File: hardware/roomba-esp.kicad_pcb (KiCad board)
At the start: 2 copper layers, 45 x 32.5 mm, 7 parts, among them P1 CONN_01X07, P2 CONN_02X10, U1 ESP-12E, U2 LM2596_module

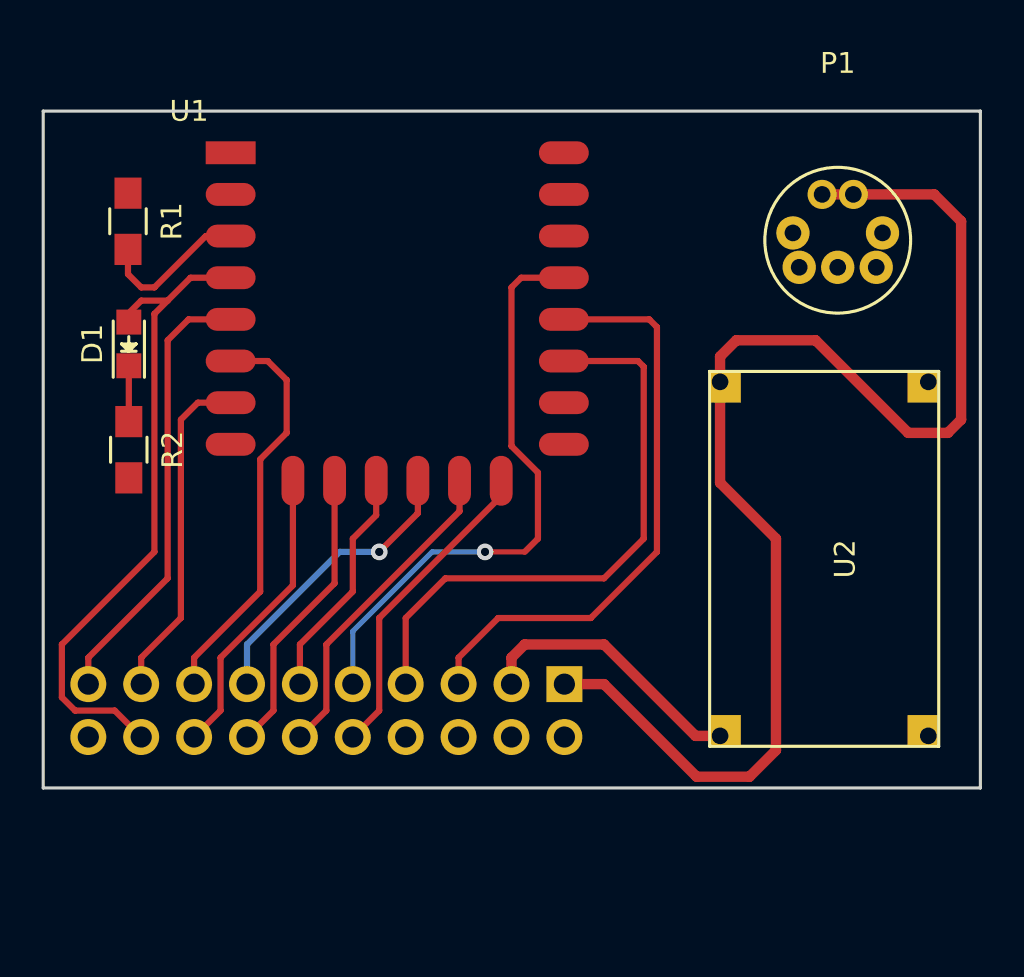
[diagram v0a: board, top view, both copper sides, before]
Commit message: finalised rev0 pcb
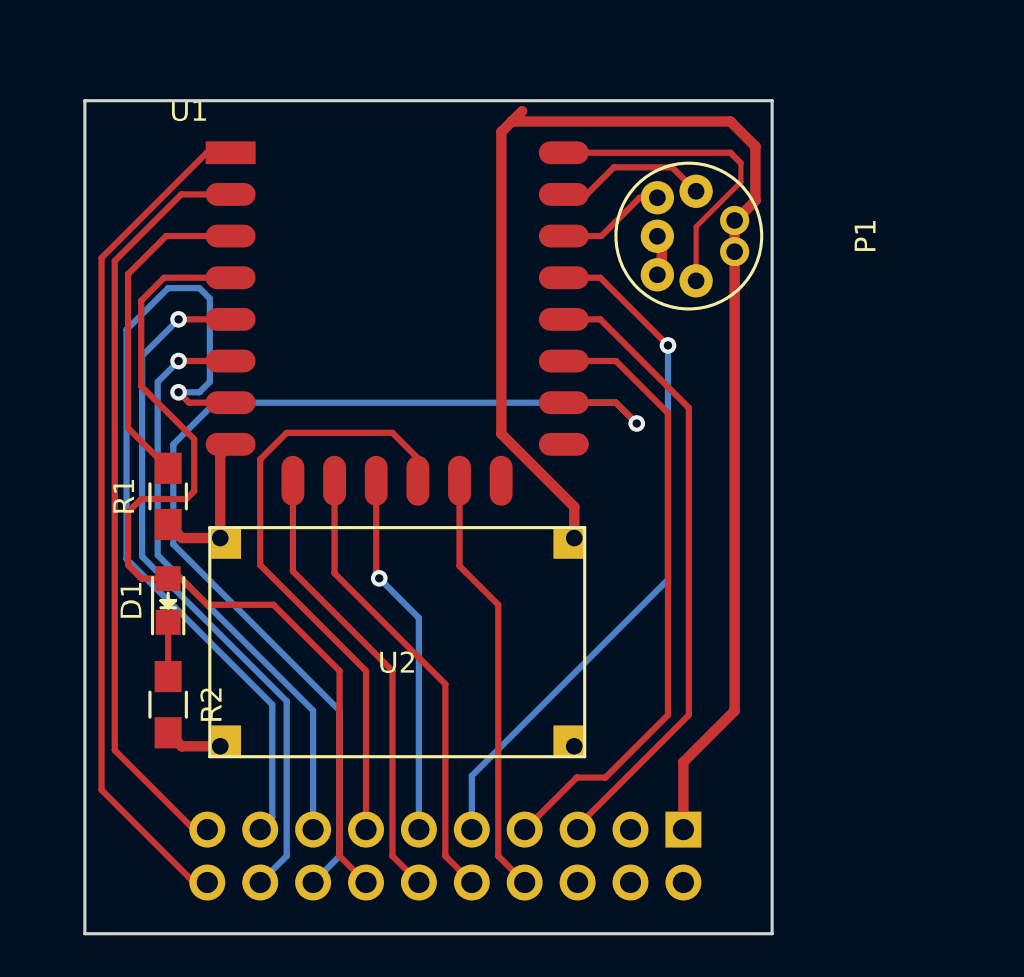
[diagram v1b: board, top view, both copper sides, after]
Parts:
- P1: footprint mini din:mini din 7 -> mini din:mini_DIN_7
- moved U2 20.9 mm to (192.0, 118.0), turned to 0 degrees
- moved R1 13.4 mm to (181.0, 111.0), turned to 90 degrees
- moved D1 12.5 mm to (181.0, 116.0)
- moved R2 12.4 mm to (181.0, 121.0)
- moved P2 9.03 mm to (205.7, 127.0)
- moved P1 7.85 mm to (214.0, 98.5), turned to 90 degrees
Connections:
- P2 pad 10: /SCK -> /MISO
- P2 pad 12: /MOSI -> /CS0
- P2 pad 14: /MISO -> /GPIO16
- P2 pad 16: /CS0 -> /GPIO15
- P2 pad 18: /GPIO16 -> /GPIO14
- P2 pad 19: /GPIO14 -> /ADC
- P2 pad 20: /GPIO15 -> /RESET
- P2 pad 6: /ADC -> /SCK
- P2 pad 8: /RESET -> /MOSI
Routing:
- net /GPIO15: track 0.00 -> 52.3 mm, vias 0 -> 1
- net /RESET: track 0.00 -> 40.8 mm
- net /ADC: track 0.00 -> 36.4 mm
- net /GPIO13: track 16.2 -> 40.6 mm, vias 0 -> 1
- net /TX: track 0.00 -> 16.0 mm
- net /GPIO10: track 14.3 -> 29.6 mm, vias 1 -> 0
- net /SCK: track 15.3 -> 0.00 mm
- net /GPIO16: track 31.8 -> 44.0 mm
- net /GPIO14: track 21.5 -> 33.7 mm, vias 0 -> 1
- net /GPIO12: track 19.5 -> 28.5 mm, vias 0 -> 1
- net Net-(R1-Pad2): track 7.40 -> 15.8 mm
- net /MISO: track 14.0 -> 22.4 mm
- net /CS0: track 14.3 -> 22.2 mm
- net /RX: track 0.00 -> 7.36 mm
- net /DD: track 0.00 -> 7.20 mm
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- added copper zone on F.Cu, net GND
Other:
- board size 45 x 32.5 mm -> 33 x 40 mm
- net class Power: clearance 0.3 -> 0.25
